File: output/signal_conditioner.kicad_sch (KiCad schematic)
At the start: 3 parts

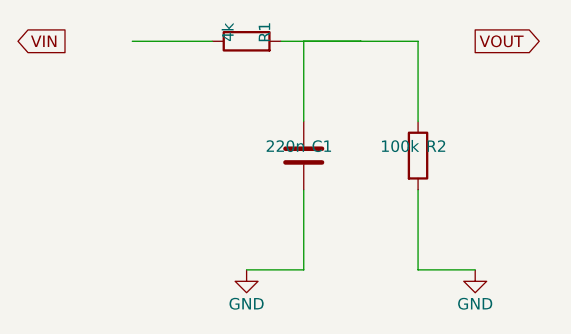
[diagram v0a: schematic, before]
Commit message: feat: revise pipeline
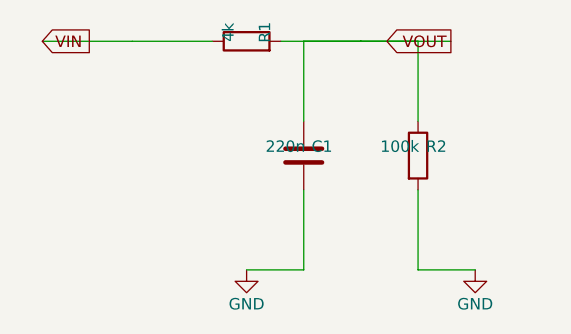
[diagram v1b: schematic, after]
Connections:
- net VIN: now also R1.1
- net VOUT: now also C1.1, R1.2, R2.1
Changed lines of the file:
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@@
     (instances
       (project "schematic"
-        (path "/df601bb8-62e9-4963-aebd-6cc9d662ebfd"
+        (path "/1d0e848e-ee1b-4645-9321-6a5002ce66ca"
           (reference "R1")
           (unit 1)
@@
     (instances
       (project "schematic"
-        (path "/df601bb8-62e9-4963-aebd-6cc9d662ebfd"
+        (path "/1d0e848e-ee1b-4645-9321-6a5002ce66ca"
           (reference "C1")
           (unit 1)
@@
     (instances
       (project "schematic"
-        (path "/df601bb8-62e9-4963-aebd-6cc9d662ebfd"
+        (path "/1d0e848e-ee1b-4645-9321-6a5002ce66ca"
           (reference "R2")
           (unit 1)
@@
     (instances
       (project "schematic"
-        (path "/df601bb8-62e9-4963-aebd-6cc9d662ebfd"
+        (path "/1d0e848e-ee1b-4645-9321-6a5002ce66ca"
           (reference "#PWR01")
           (unit 1)
@@
     (instances
       (project "schematic"
-        (path "/df601bb8-62e9-4963-aebd-6cc9d662ebfd"
+        (path "/1d0e848e-ee1b-4645-9321-6a5002ce66ca"
           (reference "#PWR02")
           (unit 1)
@@
   (global_label "VIN"
     (shape input)
-    (at 137.3 100.0 0)
+    (at 140.0 100.0 0)
     (fields_autoplaced yes)
     (effects (font (size 1.27 1.27)))
@@
   (global_label "VOUT"
     (shape output)
-    (at 188.1 100.0 0)
+    (at 185.4 100.0 180)
     (fields_autoplaced yes)
     (effects (font (size 1.27 1.27)))
@@
     (stroke (width 0) (type default))
   )
+  (wire
+    (pts (xy 140.0 100.0) (xy 150.0 100.0))
+    (stroke (width 0) (type default))
+  )
+  (wire
+    (pts (xy 175.4 100.0) (xy 185.4 100.0))
+    (stroke (width 0) (type default))
+  )
